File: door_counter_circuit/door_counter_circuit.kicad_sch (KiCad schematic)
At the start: 12 parts

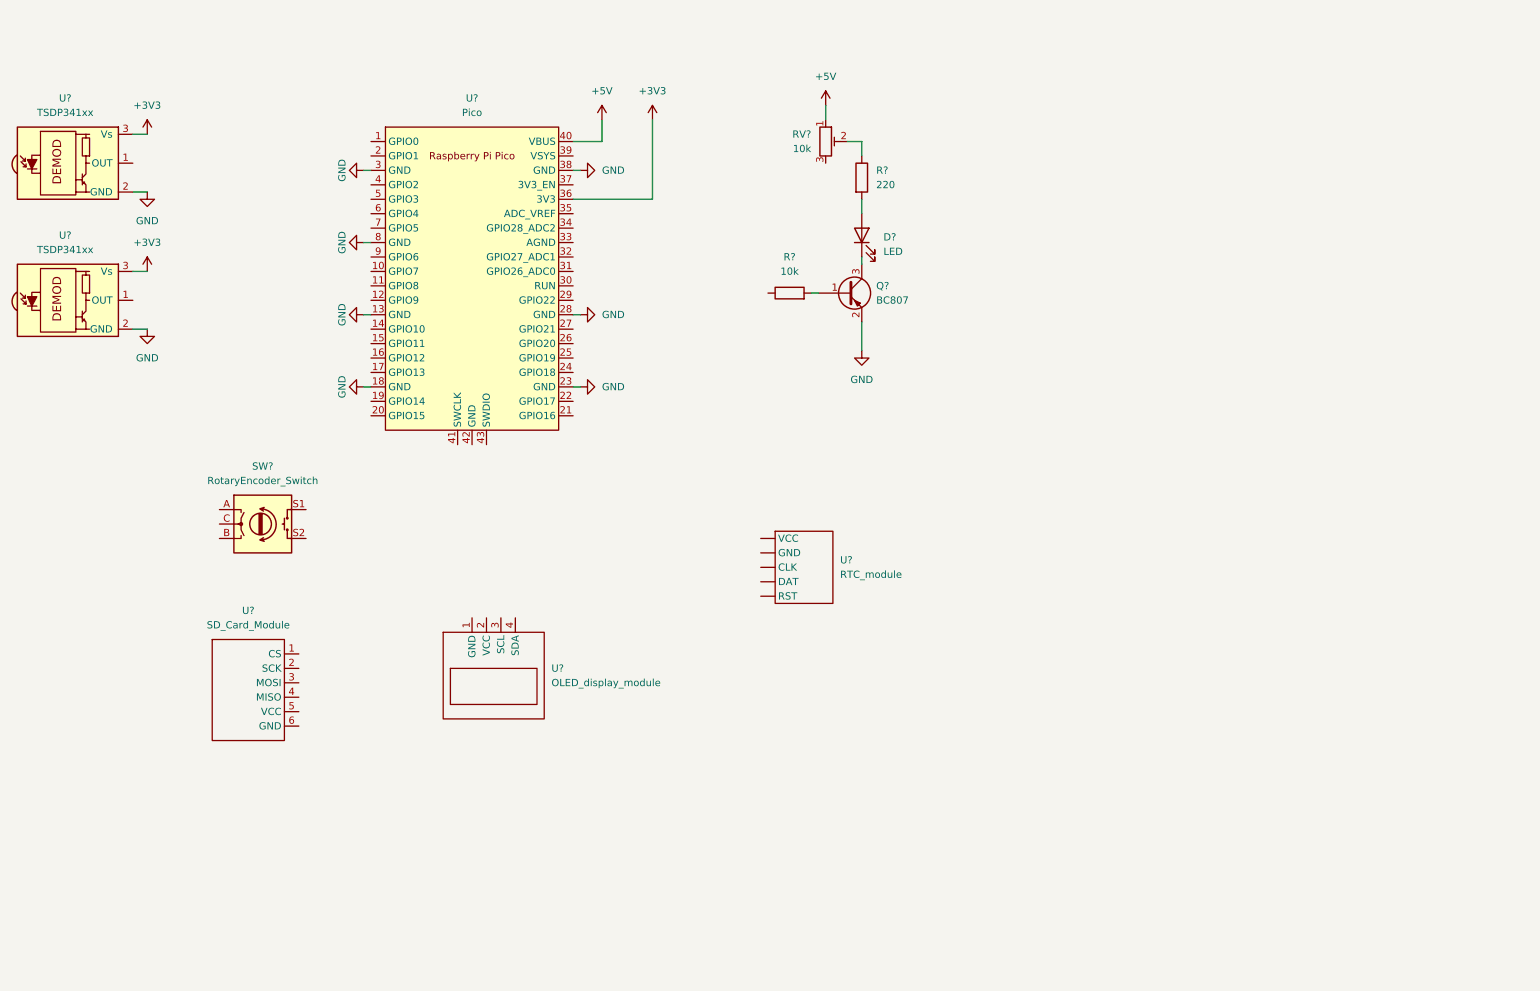
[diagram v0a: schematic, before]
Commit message: circuit board drafted
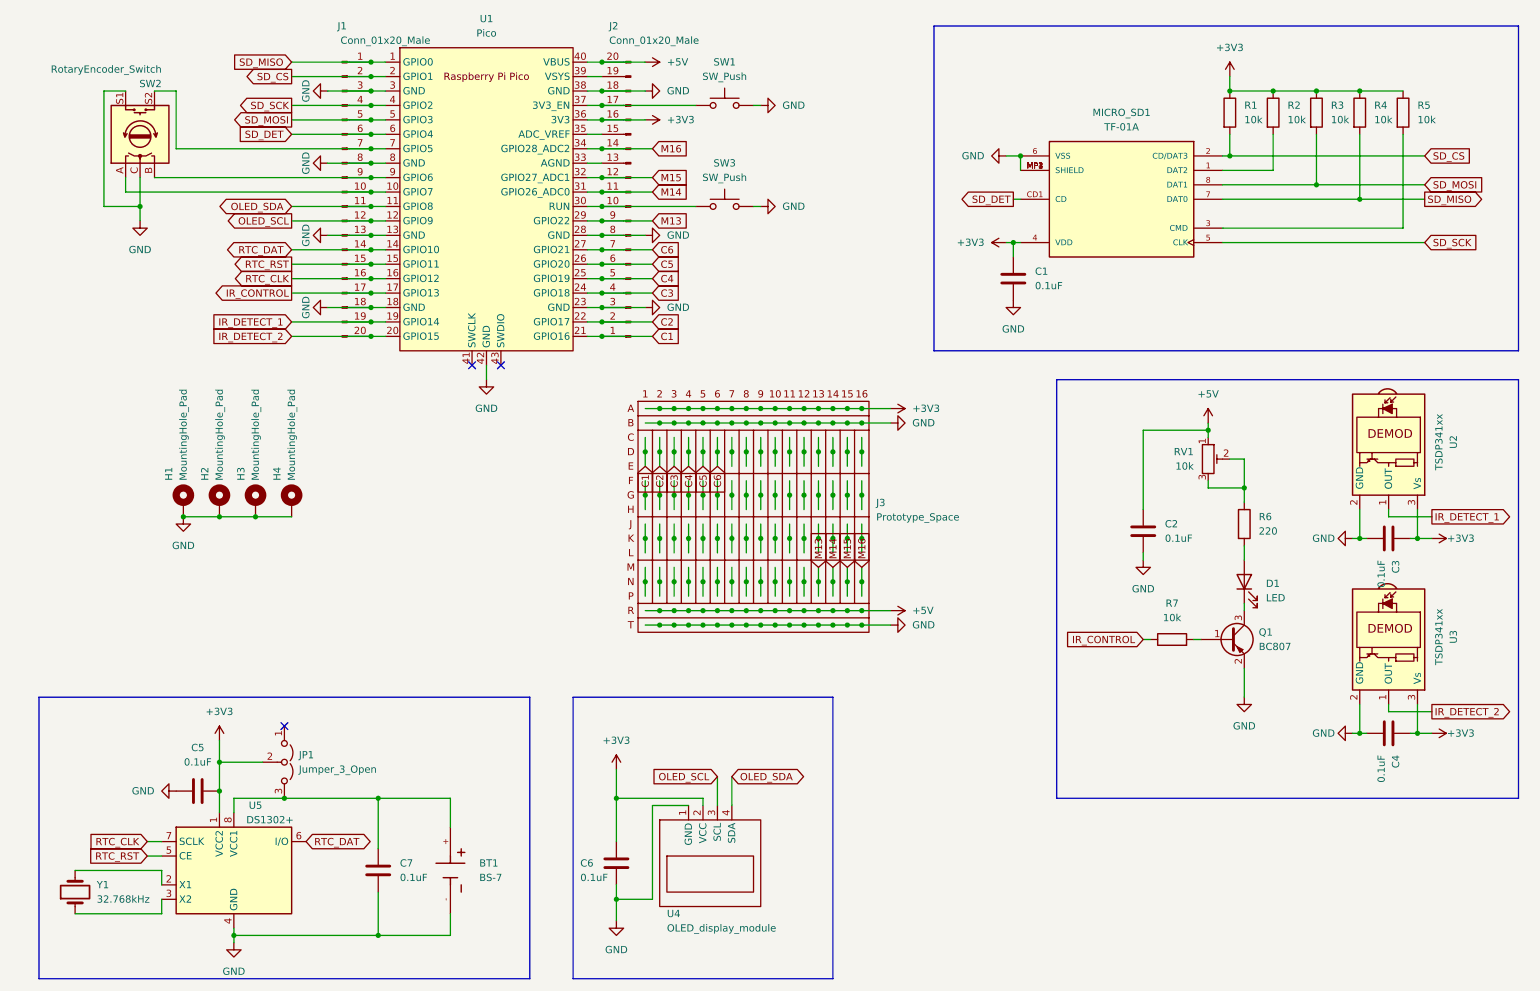
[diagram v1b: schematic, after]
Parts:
- removed U?: TSDP341xx, OptoDevice:Vishay_MOLD-3Pin, symbol Interface_Optical:TSDP341xx
- removed U?: RTC_module, symbol modules:RTC_module
- removed U?: SD_Card_Module, symbol modules:SD_Card_Module
- added BT1: BS-7, bs-7:BAT_BS-7, symbol bs-7:BS-7
- added C1, C2, C3, C4, C5, C6, C7: 0.1uF, Capacitor_SMD:C_0402_1005Metric, symbol Device:C
- added H1, H2, H3, H4: MountingHole_Pad, MountingHole:MountingHole_5mm_Pad_Via, symbol Mechanical:MountingHole_Pad
- added J1, J2: Conn_01x20_Male, Connector_PinHeader_2.54mm:PinHeader_1x20_P2.54mm_Vertical, symbol Connector:Conn_01x20_Male
- added J3: Prototype_Space, Library:Prototype Space, symbol Library:Prototype_Space
- added JP1: Jumper_3_Open, Connector_PinHeader_2.54mm:PinHeader_1x03_P2.54mm_Vertical, symbol Jumper:Jumper_3_Open
- added MICRO_SD1: TF-01A, tf01a:TF-01A, symbol tf01a:TF-01A
- added R1, R2, R3, R4, R5: 10k, Resistor_SMD:R_0603_1608Metric, symbol Device:R
- added SW1, SW3: SW_Push, Button_Switch_THT:SW_PUSH_6mm_H4.3mm, symbol Switch:SW_Push
- added U3: TSDP341xx, OptoDevice:Vishay_MOLD-3Pin, symbol Interface_Optical:TSDP341xx
- added U5: DS1302+, Package_DIP:DIP-8_W7.62mm, symbol Timer_RTC:DS1302+
- added Y1: 32.768kHz, Crystal:Crystal_C26-LF_D2.1mm_L6.5mm_Horizontal, symbol Device:Crystal
- D1: renamed from D?; footprint (none) -> LED_THT:LED_D3.0mm_Horizontal_O1.27mm_Z6.0mm
- R6, R7: renamed from R?; footprint (none) -> Resistor_SMD:R_0603_1608Metric
- RV1: renamed from RV?; footprint (none) -> Potentiometer_THT:Potentiometer_Bourns_3296W_Vertical
- SW2: renamed from SW?; footprint (none) -> Rotary_Encoder:RotaryEncoder_Alps_EC11E-Switch_Vertical_H20mm
- U1: renamed from U?; symbol RPi_Pico:Pico -> modules:Pico
- U4: renamed from U?; footprint (none) -> ssd1306:SSD1306
- gave numbers to parts that had none: 2
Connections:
- net +3V3: now also U4.2 (VCC), C1.1, C3.1, C4.1, C5.2, C6.1, J2.16 (Pin_16), J3.10A, J3.11A, J3.12A, J3.13A, J3.14A, J3.15A, J3.16A, J3.1A, J3.2A, J3.3A, J3.4A, J3.5A, J3.6A, J3.7A, J3.8A, J3.9A, JP1.2 (C), MICRO_SD1.4 (VDD), R1.1, R2.1, R3.1, R4.1, R5.1, U3.3 (Vs), U5.1 (VCC2)
- net +5V: now also C2.1, J2.20 (Pin_20), J3.10R, J3.11R, J3.12R, J3.13R, J3.14R, J3.15R, J3.16R, J3.1R, J3.2R, J3.3R, J3.4R, J3.5R, J3.6R, J3.7R, J3.8R, J3.9R
- net GND: now also SW2.C, SW2.S1, U1.42 (GND), U4.1 (GND), BT1.-, C1.2, C2.2, C3.2, C4.2, C5.1, C6.2, C7.2, H1.1, H2.1, H3.1, H4.1, J1.13 (Pin_13), J1.18 (Pin_18), J1.3 (Pin_3), J1.8 (Pin_8), J2.18 (Pin_18), J2.3 (Pin_3), J2.8 (Pin_8), J3.10B, J3.10T, J3.11B, J3.11T, J3.12B, J3.12T, J3.13B, J3.13T, J3.14B, J3.14T, J3.15B, J3.15T, J3.16B, J3.16T, J3.1B, J3.1T, J3.2B, J3.2T, J3.3B, J3.3T, J3.4B, J3.4T, J3.5B, J3.5T, J3.6B, J3.6T, J3.7B, J3.7T, J3.8B, J3.8T, J3.9B, J3.9T, MICRO_SD1.6 (VSS), MICRO_SD1.MP1 (SHIELD), MICRO_SD1.MP2 (SHIELD), MICRO_SD1.MP3 (SHIELD), MICRO_SD1.MP4 (SHIELD), SW1.2, SW3.2, U3.2 (GND), U5.4 (GND)
- net at R6.1, RV1.2: now also RV1.3
- net at SW2.A: now also U1.10 (GPIO7), J1.10 (Pin_10)
- net at SW2.B: now also U1.9 (GPIO6), J1.9 (Pin_9)
- net at SW2.S2: now also U1.7 (GPIO5), J1.7 (Pin_7)
- net SD_MISO: now reaches U1.1 (GPIO0)
- net SD_MISO: now also J1.1 (Pin_1), MICRO_SD1.7 (DAT0), R4.2
- net OLED_SDA: now reaches U1.11 (GPIO8)
- net OLED_SDA: now also U4.4 (SDA), J1.11 (Pin_11)
- net OLED_SCL: now reaches U1.12 (GPIO9)
- net OLED_SCL: now also U4.3 (SCL), J1.12 (Pin_12)
- net RTC_DAT: now reaches U1.14 (GPIO10)
- net RTC_DAT: now also J1.14 (Pin_14), U5.6 (I/O)
- net RTC_RST: now reaches U1.15 (GPIO11)
- net RTC_RST: now also J1.15 (Pin_15), U5.5 (CE)
- net RTC_CLK: now reaches U1.16 (GPIO12)
- net RTC_CLK: now also J1.16 (Pin_16), U5.7 (SCLK)
- net IR_CONTROL: now reaches U1.17 (GPIO13)
- net IR_CONTROL: now also R7.1, J1.17 (Pin_17)
- net IR_DETECT_1: now reaches U1.19 (GPIO14)
- net IR_DETECT_1: now also U2.1 (OUT), J1.19 (Pin_19)
- net SD_CS: now reaches U1.2 (GPIO1)
- net SD_CS: now also J1.2 (Pin_2), MICRO_SD1.2 (CD/DAT3), R1.2
- net IR_DETECT_2: now reaches U1.20 (GPIO15)
- net IR_DETECT_2: now also J1.20 (Pin_20), U3.1 (OUT)
- net C1: now reaches U1.21 (GPIO16)
- net C1: now also J2.1 (Pin_1), J3.1C, J3.1D, J3.1E
- net C2: now reaches U1.22 (GPIO17)
- net C2: now also J2.2 (Pin_2), J3.2C, J3.2D, J3.2E
- net C3: now reaches U1.24 (GPIO18)
- net C3: now also J2.4 (Pin_4), J3.3C, J3.3D, J3.3E
- net C4: now reaches U1.25 (GPIO19)
- net C4: now also J2.5 (Pin_5), J3.4C, J3.4D, J3.4E
- net C5: now reaches U1.26 (GPIO20)
- net C5: now also J2.6 (Pin_6), J3.5C, J3.5D, J3.5E
- net C6: now reaches U1.27 (GPIO21)
- net C6: now also J2.7 (Pin_7), J3.6C, J3.6D, J3.6E
- net M13: now reaches U1.29 (GPIO22)
- net M13: now also J2.9 (Pin_9), J3.13M, J3.13N, J3.13P
- net at U1.30 (RUN): now also J2.10 (Pin_10), SW3.1
- net M14: now reaches U1.31 (GPIO26_ADC0)
- net M14: now also J2.11 (Pin_11), J3.14M, J3.14N, J3.14P
- net M15: now reaches U1.32 (GPIO27_ADC1)
- net M15: now also J2.12 (Pin_12), J3.15M, J3.15N, J3.15P
- net at U1.33 (AGND): now also J2.13 (Pin_13)
- net M16: now reaches U1.34 (GPIO28_ADC2)
- net M16: now also J2.14 (Pin_14), J3.16M, J3.16N, J3.16P
- net at U1.35 (ADC_VREF): now also J2.15 (Pin_15)
- net at U1.37 (3V3_EN): now also J2.17 (Pin_17), SW1.1
- net at U1.39 (VSYS): now also J2.19 (Pin_19)
- net SD_SCK: now reaches U1.4 (GPIO2)
- net SD_SCK: now also J1.4 (Pin_4), MICRO_SD1.5 (CLK)
- net SD_MOSI: now reaches U1.5 (GPIO3)
- net SD_MOSI: now also J1.5 (Pin_5), MICRO_SD1.8 (DAT1), R3.2
- net SD_DET: now reaches U1.6 (GPIO4)
- net SD_DET: now also J1.6 (Pin_6), MICRO_SD1.CD1 (CD)
- new net: BT1.+, C7.1, JP1.3 (B), U5.8 (VCC1)
- new net: U5.3 (X2), Y1.1
- new net: U5.2 (X1), Y1.2
- new net: MICRO_SD1.1 (DAT2), R2.2
- new net: MICRO_SD1.3 (CMD), R5.2
- new net: J3.10C, J3.10D, J3.10E
- new net: J3.10F, J3.10G, J3.10H
- new net: J3.10J, J3.10K, J3.10L
- new net: J3.10M, J3.10N, J3.10P
- new net: J3.11C, J3.11D, J3.11E
- new net: J3.11F, J3.11G, J3.11H
- new net: J3.11J, J3.11K, J3.11L
- new net: J3.11M, J3.11N, J3.11P
- new net: J3.12C, J3.12D, J3.12E
- new net: J3.12F, J3.12G, J3.12H
- new net: J3.12J, J3.12K, J3.12L
- new net: J3.12M, J3.12N, J3.12P
- new net: J3.13C, J3.13D, J3.13E
- new net: J3.13F, J3.13G, J3.13H
- new net: J3.13J, J3.13K, J3.13L
- new net: J3.14C, J3.14D, J3.14E
- new net: J3.14F, J3.14G, J3.14H
- new net: J3.14J, J3.14K, J3.14L
- new net: J3.15C, J3.15D, J3.15E
- new net: J3.15F, J3.15G, J3.15H
- new net: J3.15J, J3.15K, J3.15L
- new net: J3.16C, J3.16D, J3.16E
- new net: J3.16F, J3.16G, J3.16H
- new net: J3.16J, J3.16K, J3.16L
- new net: J3.1F, J3.1G, J3.1H
- new net: J3.1J, J3.1K, J3.1L
- new net: J3.1M, J3.1N, J3.1P
- new net: J3.2F, J3.2G, J3.2H
- new net: J3.2J, J3.2K, J3.2L
- new net: J3.2M, J3.2N, J3.2P
- new net: J3.3F, J3.3G, J3.3H
- new net: J3.3J, J3.3K, J3.3L
- new net: J3.3M, J3.3N, J3.3P
- new net: J3.4F, J3.4G, J3.4H
- new net: J3.4J, J3.4K, J3.4L
- new net: J3.4M, J3.4N, J3.4P
- new net: J3.5F, J3.5G, J3.5H
- new net: J3.5J, J3.5K, J3.5L
- new net: J3.5M, J3.5N, J3.5P
- new net: J3.6F, J3.6G, J3.6H
- new net: J3.6J, J3.6K, J3.6L
- new net: J3.6M, J3.6N, J3.6P
- new net: J3.7C, J3.7D, J3.7E
- new net: J3.7F, J3.7G, J3.7H
- new net: J3.7J, J3.7K, J3.7L
- new net: J3.7M, J3.7N, J3.7P
- new net: J3.8C, J3.8D, J3.8E
- new net: J3.8F, J3.8G, J3.8H
- new net: J3.8J, J3.8K, J3.8L
- new net: J3.8M, J3.8N, J3.8P
- new net: J3.9C, J3.9D, J3.9E
- new net: J3.9F, J3.9G, J3.9H
- new net: J3.9J, J3.9K, J3.9L
- new net: J3.9M, J3.9N, J3.9P
- no-connect marks 0 -> 3
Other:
- moved on the sheet: D1, Q1, R6, R7, RV1, SW2, U1, U2, U4
